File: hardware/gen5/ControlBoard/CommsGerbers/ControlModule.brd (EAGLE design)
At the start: 38.5 x 64.9 mm, 44 parts, among them Q1 BSS123, Q2 BSS123, U1 ATMEGA328P-AU

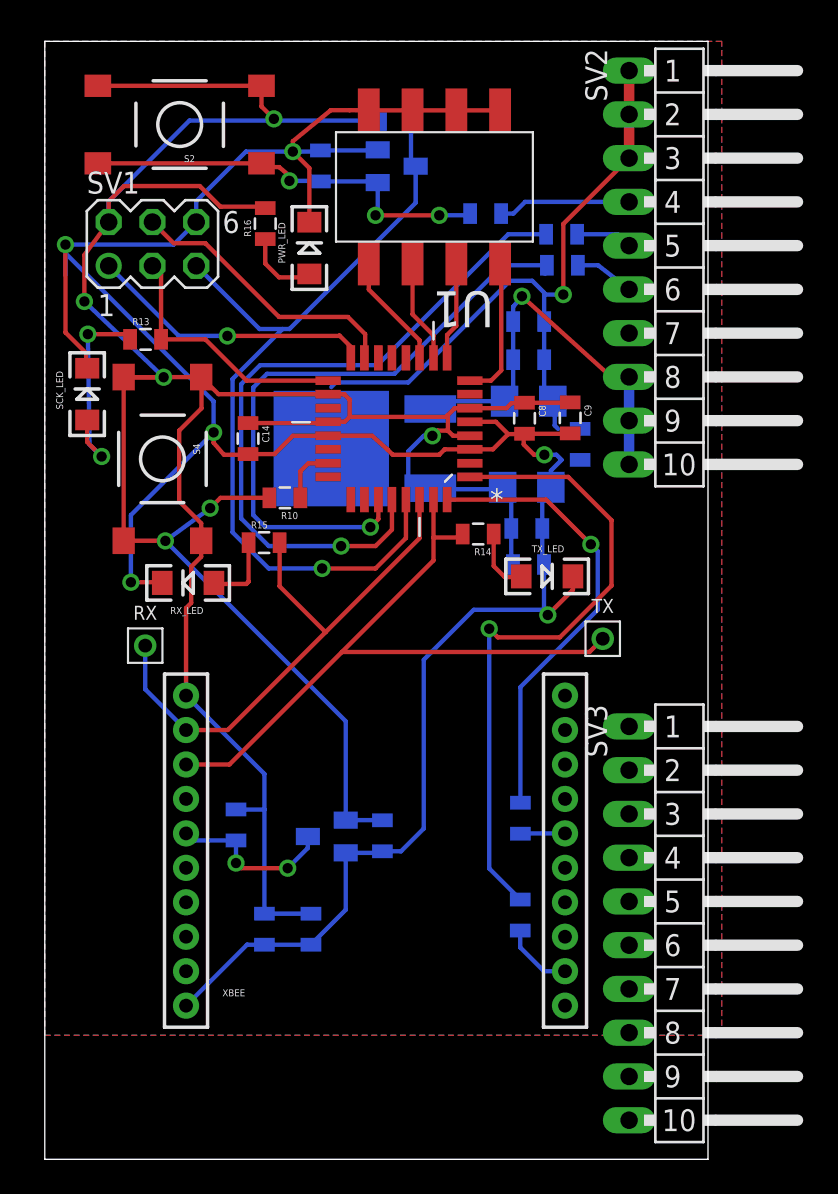
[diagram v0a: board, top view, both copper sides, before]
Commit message: added comms board gerbers
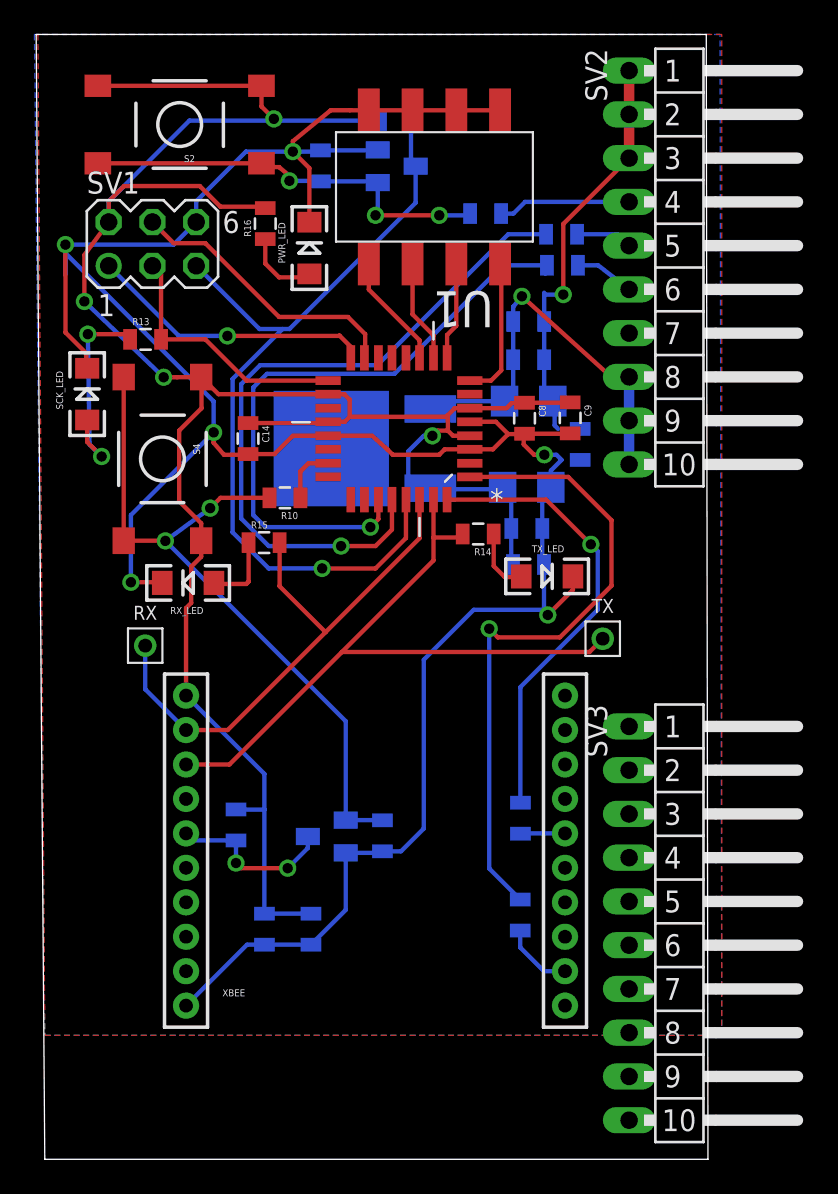
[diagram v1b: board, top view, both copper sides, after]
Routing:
- net 12VGND: track 39.1 -> 23.9 mm
- net 3.3V: track 145.8 -> 142.1 mm
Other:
- board size 38.5 x 64.9 mm -> 39 x 65.3 mm
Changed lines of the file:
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@@
 <plain>
 <wire x1="0" y1="0" x2="38.5" y2="0" width="0" layer="20"/>
-<wire x1="38.5" y1="0" x2="38.5" y2="64.9" width="0" layer="20"/>
-<wire x1="38.5" y1="64.9" x2="0" y2="64.9" width="0" layer="20"/>
-<wire x1="0" y1="64.9" x2="0" y2="0" width="0" layer="20"/>
+<wire x1="38.5" y1="0" x2="38.4" y2="65.3" width="0" layer="20"/>
+<wire x1="38.4" y1="65.3" x2="-0.5" y2="65.3" width="0" layer="20"/>
+<wire x1="-0.5" y1="65.3" x2="0" y2="0" width="0" layer="20"/>
 <text x="-13.6" y="68.5" size="1.778" layer="48">Might need to be condensed further. I have some ideas if necessary.</text>
 </plain>
@@
 <wire x1="11.1" y1="20.31" x2="11.11" y2="20.3" width="0.254" layer="16"/>
 <wire x1="11.11" y1="20.3" x2="12.75" y2="20.3" width="0.254" layer="16"/>
-<wire x1="9.08" y1="45.41" x2="5.07" y2="45.4" width="0.254" layer="1"/>
-<wire x1="5.07" y1="45.4" x2="6.9" y2="45.4" width="0.254" layer="1"/>
+<wire x1="9.08" y1="45.41" x2="7.67" y2="45.4" width="0.254" layer="1"/>
+<wire x1="7.67" y1="45.4" x2="6.9" y2="45.4" width="0.254" layer="1"/>
 <wire x1="9.08" y1="35.91" x2="9.08" y2="36.92" width="0.254" layer="1"/>
 <wire x1="9.08" y1="36.92" x2="7.8" y2="38.2" width="0.254" layer="1"/>
@@
 <wire x1="28.99" y1="46.42" x2="28.99" y2="44.51" width="0.254" layer="16"/>
 <wire x1="28.99" y1="44.51" x2="29.49" y2="44.01" width="0.254" layer="16"/>
-<wire x1="16.63" y1="44.83" x2="16.9" y2="45.1" width="0.254" layer="16"/>
-<wire x1="16.9" y1="45.1" x2="21.1" y2="45.1" width="0.254" layer="16"/>
-<wire x1="21.1" y1="45.1" x2="27" y2="51" width="0.254" layer="16"/>
-<wire x1="27" y1="51" x2="28.3" y2="51" width="0.254" layer="16"/>
-<wire x1="28.3" y1="51" x2="28.99" y2="50.31" width="0.254" layer="16"/>
 <wire x1="28.99" y1="50.31" x2="28.99" y2="50.2" width="0.254" layer="16"/>
 <contactref element="SV2" pad="1"/>
@@
 <vertex x="0" y="7.2"/>
 <vertex x="39.3" y="7.2"/>
-<vertex x="39.3" y="64.9"/>
-<vertex x="0" y="64.9"/>
+<vertex x="39.3" y="65.3"/>
+<vertex x="-0.4" y="65.3"/>
 </polygon>
 </signal>
@@
 <vertex x="0" y="7.2"/>
 <vertex x="39.3" y="7.2"/>
-<vertex x="39.3" y="64.9"/>
-<vertex x="0" y="64.9"/>
+<vertex x="39.2" y="65.3"/>
+<vertex x="-0.6" y="65.3"/>
 </polygon>
 </signal>
